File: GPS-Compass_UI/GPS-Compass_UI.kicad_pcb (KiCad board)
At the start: 2 copper layers, 20 x 95 mm, 29 parts, among them J1 FFC2B28-12-G, SW1 SPDT, SW2 SW_SPDT, SW3 EXT, SW4 RESET, SW5 RESET, SW6 EXT, SW7 EXT, SW8 EXT

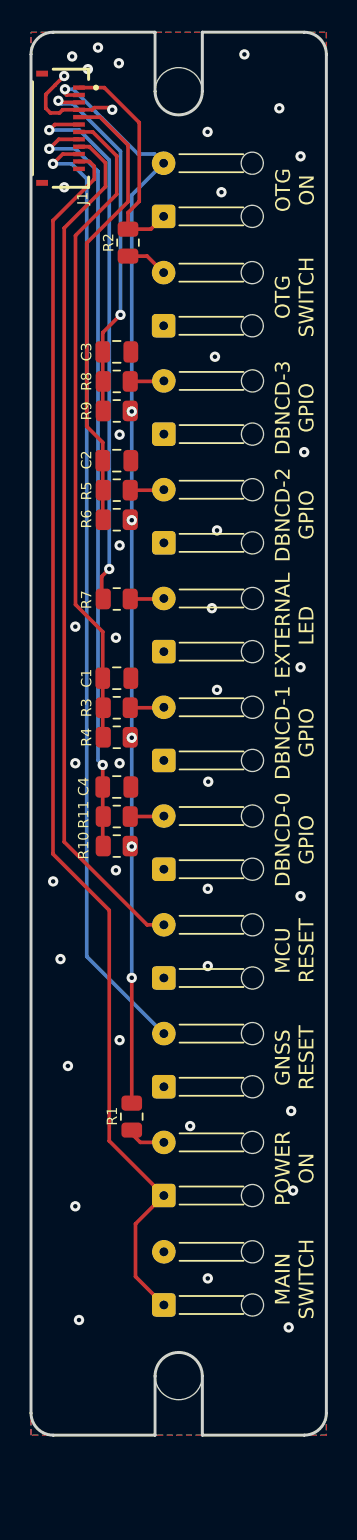
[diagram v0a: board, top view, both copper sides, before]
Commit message: asdasd
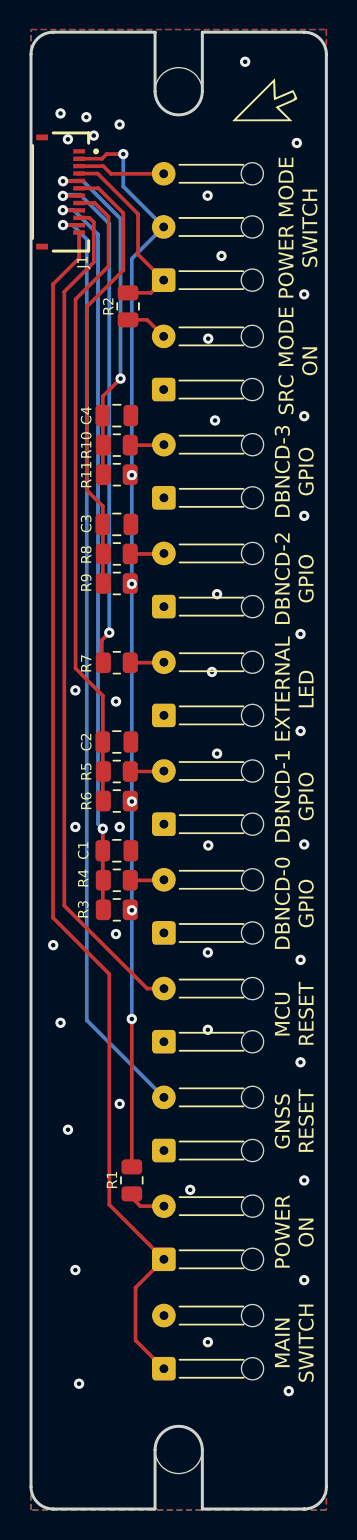
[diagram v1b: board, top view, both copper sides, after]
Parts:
- added G***: LOGO, sumec_graphic:CURSOR_IMG, F.Cu at (206.4, 50.2)
- added G***: LOGO, sumec_graphic:APERTURE_ART, B.Cu at (198.5, 99.0)
- SW2: footprint Connector_Wire:SolderWire-0.1sqmm_1x02_P3.6mm_D0.4mm_OD1mm_Relief -> Connector_Wire:SolderWire-0.1sqmm_1x03_P3.6mm_D0.4mm_OD1mm_Relief
- moved H1 5.00 mm to (198.2, 145.0)
- moved D2 4.32 mm to (197.2, 132.1)
- moved D3 4.32 mm to (197.2, 95.3)
- moved R1 4.32 mm to (195.1, 126.7)
- moved SW1 4.32 mm to (197.2, 139.5)
- moved SW3 4.32 mm to (197.2, 117.4)
- moved SW4 4.32 mm to (197.2, 110.0)
- moved SW5 4.32 mm to (197.2, 124.7)
- moved SW6 4.32 mm to (197.2, 102.6)
- moved SW7 4.32 mm to (197.2, 87.9)
- moved SW8 4.32 mm to (197.2, 80.5)
- moved J1 4.32 mm to (190.3, 59.8)
- moved R2 4.32 mm to (194.8, 67.6)
- moved C1 4.32 mm to (194.1, 104.4)
- moved C2 4.32 mm to (194.1, 97.1)
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- renumbered C4 to C1, C1 to C2, C2 to C3, C3 to C4, R8 to R10, R9 to R11, R10 to R3, R11 to R4, R3 to R5, R4 to R6, R5 to R8, R6 to R9, SW4 to SW3, SW8 to SW4, SW3 to SW6, SW6 to SW7, SW7 to SW8
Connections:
- J1 pad 1: /OTG_ON -> GND
- J1 pad 10: /GNSS_RST -> /EN
- J1 pad 11: /MSW_ON -> /GNSS_RST
- J1 pad 12: unconnected-(J1-Pad12) -> /MSW_ON
- J1 pad 3: /DBNCD_3 -> /SINK-MODE
- J1 pad 4: GND -> /SRC-MODE
- J1 pad 5: /DBNCD_2 -> /DBNCD_3
- J1 pad 6: /LED_EXT -> /DBNCD_2
- J1 pad 7: /DBNCD_1 -> /LED_EXT
- J1 pad 8: /DBNCD_0 -> /DBNCD_1
- J1 pad 9: /EN -> /DBNCD_0
- R2 pad 1: /OTG_ON -> /SRC-MODE
- SW2 pad 1: /OTG_ON -> /SRC-MODE
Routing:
- net /OTG_ON: track 15.4 -> 0.00 mm
- net /SRC-MODE: track 0.00 -> 13.1 mm
- net GND: track 7.55 -> 0.00 mm, vias 40 -> 41
- net /SINK-MODE: track 0.00 -> 5.95 mm
- net /DBNCD_0: track 52.1 -> 50.1 mm
- net /LED_EXT: track 37.0 -> 35.1 mm
- net /MSW_ON: track 84.1 -> 82.4 mm
- net /GNSS_RST: track 64.8 -> 63.4 mm
- net /DBNCD_3: track 25.2 -> 23.9 mm
- net /EN: track 58.5 -> 57.3 mm
- net /DBNCD_1: track 44.5 -> 43.6 mm
- net +3V3: track 75.2 -> 74.4 mm
- net /DBNCD_2: track 31.1 -> 30.3 mm
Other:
- board size 20 x 95 mm -> 20 x 100 mm
- board text added: "POWER MODE SWITCH"
- board text added: "SRC MODE ON"
- board text removed: "OTG ON"
- board text removed: "OTG SWITCH"

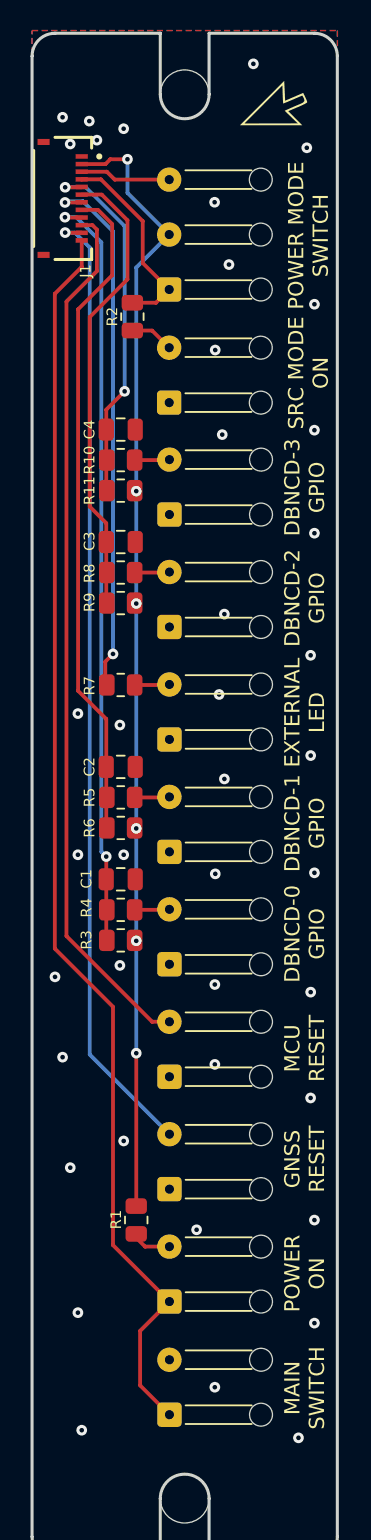
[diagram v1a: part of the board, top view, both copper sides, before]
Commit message: i think im depressed again
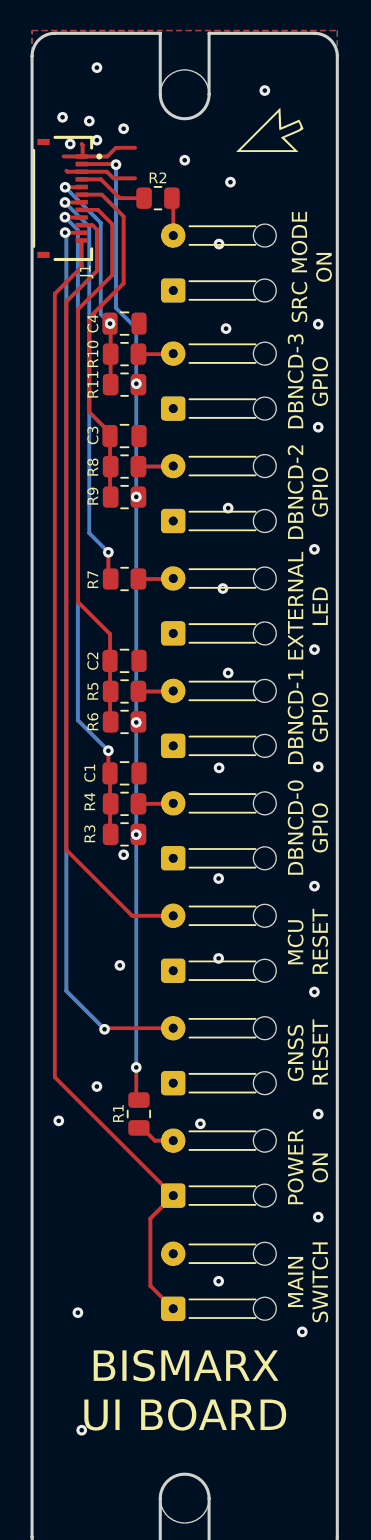
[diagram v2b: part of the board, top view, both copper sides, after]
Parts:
- removed SW2: SW_SPDT, Connector_Wire:SolderWire-0.1sqmm_1x03_P3.6mm_D0.4mm_OD1mm_Relief
- moved R2 7.94 mm to (196.5, 59.8), turned to 0 degrees
- moved D1 7.35 mm to (197.5, 65.8)
- moved D2 6.95 mm to (197.5, 125.1)
- moved D3 6.95 mm to (197.5, 88.3)
- moved SW1 6.95 mm to (197.5, 132.6)
- moved SW3 6.95 mm to (197.5, 110.4)
- moved SW4 6.95 mm to (197.5, 103.0)
- moved SW5 6.95 mm to (197.5, 117.8)
- moved SW6 6.95 mm to (197.5, 95.7)
- moved SW7 6.95 mm to (197.5, 81.0)
- moved SW8 6.95 mm to (197.5, 73.6)
- moved C1 6.95 mm to (194.3, 97.5)
- moved C2 6.95 mm to (194.3, 90.1)
- moved C3 6.95 mm to (194.3, 75.4)
- moved C4 6.95 mm to (194.3, 68.0)
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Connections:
- net /SRC-MODE renamed /OTG
- J1 pad 3: /SINK-MODE -> GND
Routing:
- net GND: track 0.00 -> 10.5 mm, vias 41 -> 35
- net +3V3: track 74.4 -> 65.0 mm
- net /DBNCD_3: track 23.9 -> 15.3 mm
- net /OTG: track 13.1 -> 4.93 mm
- net /LED_EXT: track 35.1 -> 27.2 mm
- net /DBNCD_0: track 50.1 -> 42.8 mm
- net /MSW_ON: track 82.4 -> 75.2 mm
- net /DBNCD_2: track 30.3 -> 23.3 mm
- net /DBNCD_1: track 43.6 -> 37.7 mm
- net /SINK-MODE: track 5.95 -> 0.00 mm
- net /EN: track 57.3 -> 51.4 mm
- net /GNSS_RST: track 63.4 -> 58.9 mm, vias 1 -> 2
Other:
- board text added: "BISMARX UI BOARD"
- board text removed: "POWER MODE SWITCH"

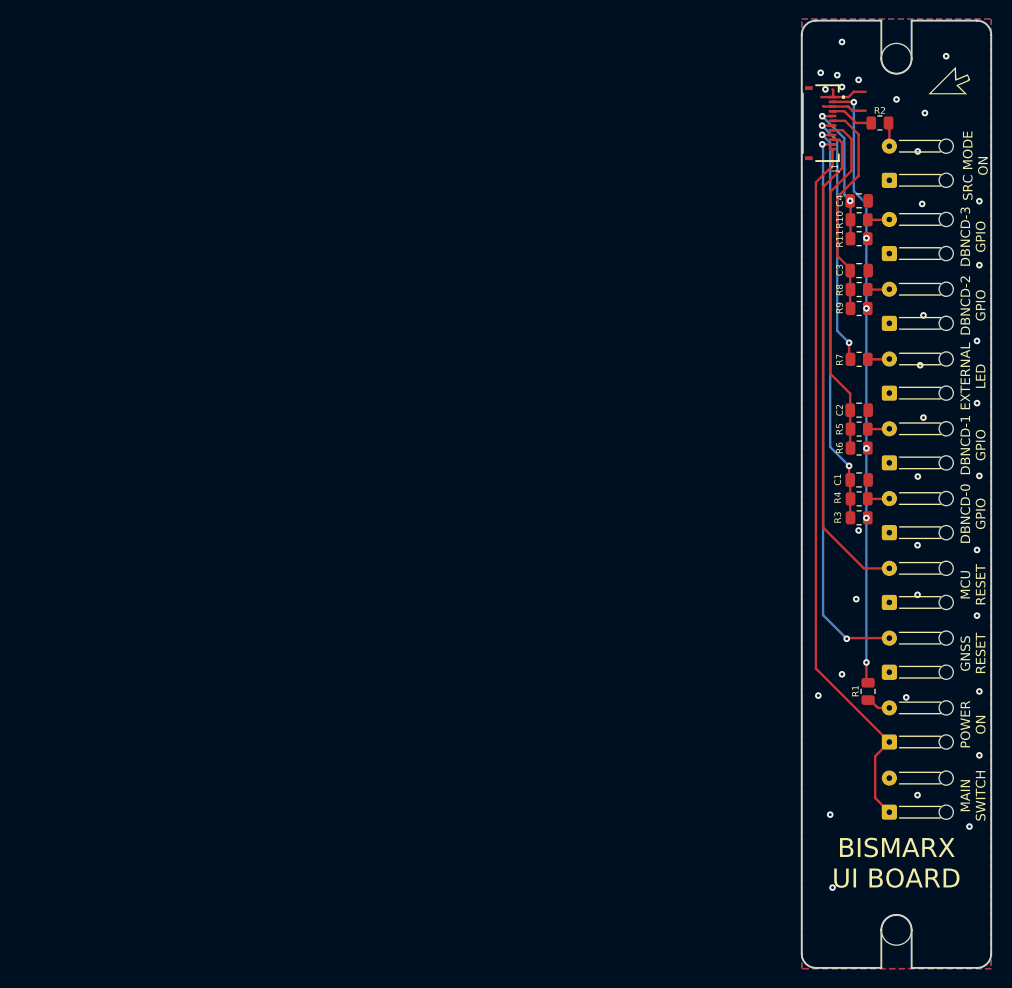
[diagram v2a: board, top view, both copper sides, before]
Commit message: asdasd
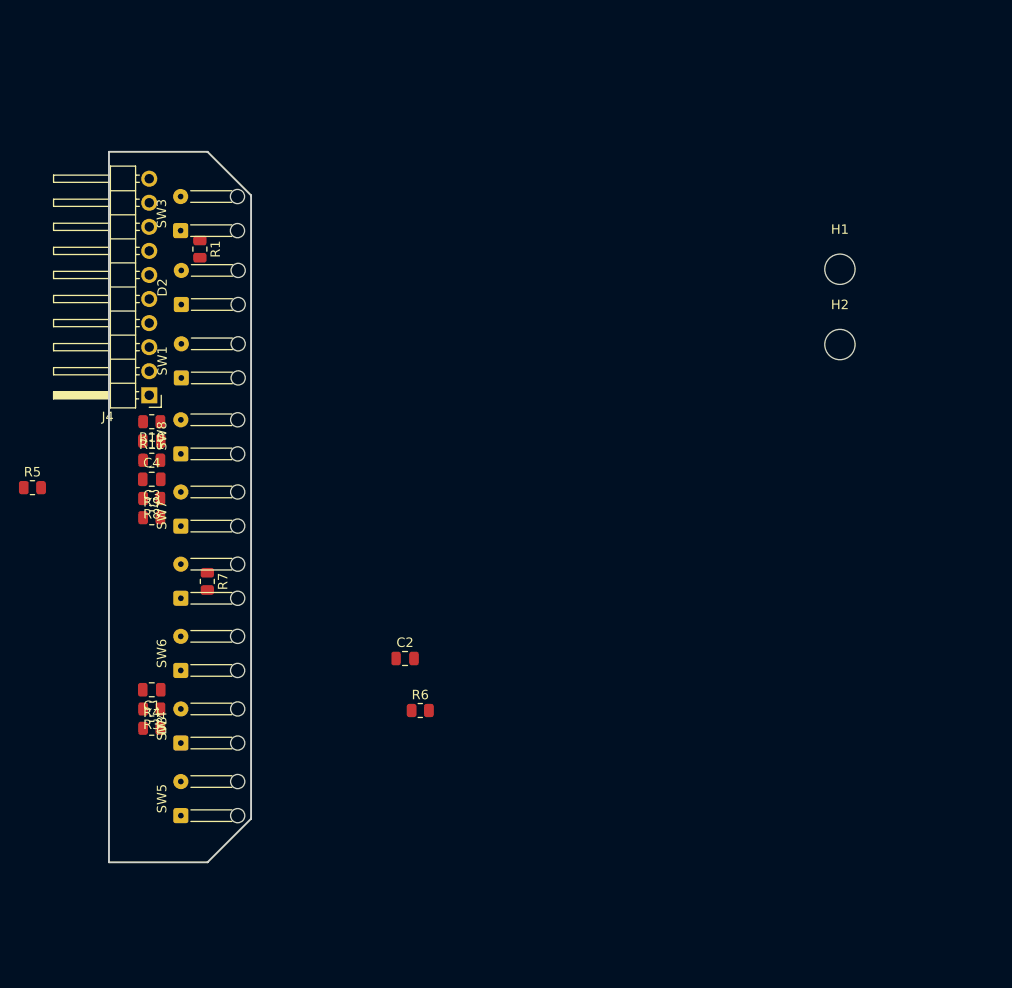
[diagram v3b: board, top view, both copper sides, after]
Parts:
- removed D1: LED, Connector_Wire:SolderWire-0.1sqmm_1x02_P3.6mm_D0.4mm_OD1mm_Relief
- removed G***: LOGO, sumec_graphic:CURSOR_IMG
- removed G***: LOGO, sumec_graphic:APERTURE_ART
- removed J1: FFC2B28-12-G, gps-compass_brd:GCT_FFC2B28-12-G
- removed R2: 2.2k, Resistor_SMD:R_0805_2012Metric
- added J4: Conn_01x10_Socket, Connector_PinHeader_2.54mm:PinHeader_1x10_P2.54mm_Horizontal, F.Cu at (119.4, 88.5)
- moved D2 87.9 mm to (122.8, 79.0)
- moved SW1 87.7 mm to (122.8, 86.7)
- moved R5 87.5 mm to (107.0, 98.3), turned to 0 degrees
- moved R1 84.6 mm to (124.7, 73.1)
- moved SW3 84.5 mm to (122.7, 71.2)
- moved C4 78.9 mm to (119.6, 93.4)
- moved R11 78.3 mm to (119.6, 95.4)
- moved SW4 78.0 mm to (122.7, 125.3)
- moved SW6 77.9 mm to (122.7, 117.6)
- moved R4 77.9 mm to (119.6, 123.7)
- moved R3 77.9 mm to (119.6, 121.7)
- moved C1 77.9 mm to (119.6, 119.6)
- moved R9 77.9 mm to (119.6, 101.5)
- moved D3 77.9 mm to (122.7, 110.0)
- moved R8 77.9 mm to (119.6, 99.4)
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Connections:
- SW3 pad 1: GND -> /EN
- SW3 pad 2: /EN -> GND
- SW5 pad 1: GND -> /GNSS_RST
- SW5 pad 2: /GNSS_RST -> GND
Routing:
- net /MSW_ON: track 75.2 -> 0.00 mm
- net +3V3: track 65.0 -> 0.00 mm, vias 6 -> 0
- net /GNSS_RST: track 58.9 -> 0.00 mm, vias 2 -> 0
- net /EN: track 51.4 -> 0.00 mm
- net /DBNCD_0: track 42.8 -> 0.00 mm, vias 2 -> 0
- net /DBNCD_1: track 37.7 -> 0.00 mm
- net /LED_EXT: track 27.2 -> 0.00 mm, vias 2 -> 0
- net /DBNCD_2: track 23.3 -> 0.00 mm
- net /DBNCD_3: track 15.3 -> 0.00 mm, vias 2 -> 0
- net GND: track 10.5 -> 0.00 mm, vias 35 -> 0
- net /OTG: track 4.93 -> 0.00 mm
- net Net-(D2-A): track 2.82 -> 0.00 mm
- net Net-(D1-A): track 2.49 -> 0.00 mm
- net /DB_0: track 2.34 -> 0.00 mm
- net Net-(D3-A): track 2.29 -> 0.00 mm
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- removed copper zone on B.Cu, net GND
- removed copper zone on F.Cu, net GND
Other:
- board size 20 x 100 mm -> 15 x 75 mm
- board text removed: "BISMARX UI BOARD"
- board text removed: "DBNCD-0 GPIO"
- board text removed: "DBNCD-1 GPIO"
- board text removed: "DBNCD-2 GPIO"
- board text removed: "DBNCD-3 GPIO"
- board text removed: "EXTERNAL LED"
- board text removed: "GNSS RESET"
- board text removed: "MAIN SWITCH"
- board text removed: "MCU RESET"
- board text removed: "POWER ON"
- board text removed: "SRC MODE ON"
